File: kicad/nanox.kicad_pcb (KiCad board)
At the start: 4 copper layers, 61.7 x 15.9 mm, 137 parts, among them P1 likely an ESD protection diod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, P2 likely an ESD protection diod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, P3 likely an ESD protection diod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, P4 likely an ESD protection diod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, P5 likely an ESD protection diod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, SW1 push button, left, SW2 push button, right, X1 ?, X10 unknown, marked 1C4F, likely 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, X2 unknown, marked 2GC, X3 unknown, marked 6, X4 ?, X5 ?, X6 ?, X7 ?, X8 ?, X9 unknown, marked P8W 26, Y1 crystal, likely the 32 MHz HSE

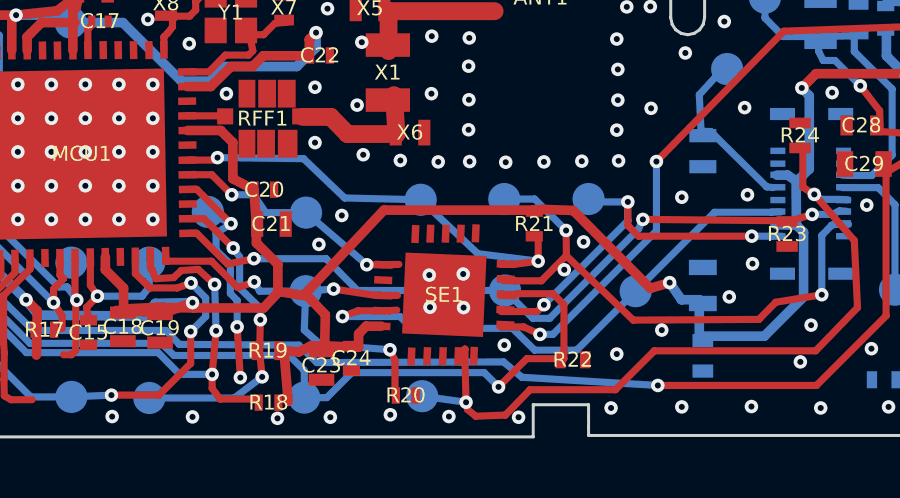
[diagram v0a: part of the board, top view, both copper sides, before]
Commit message: Put the secure element's pads on the real ones, and land its traces on them
The SE outline sat about 0.3 mm left of the real package, so OLED SPI CS
ran down the real pin 9 but stopped beside the modelled one, with a stub
across to it. The outline now follows the pads measured in the bare photo,
and every SE trace ends on its pin's centre with a straight final run;
the CS stub is gone.

Co-Authored-By: Claude Opus 5.5 <noreply@anthropic.com>
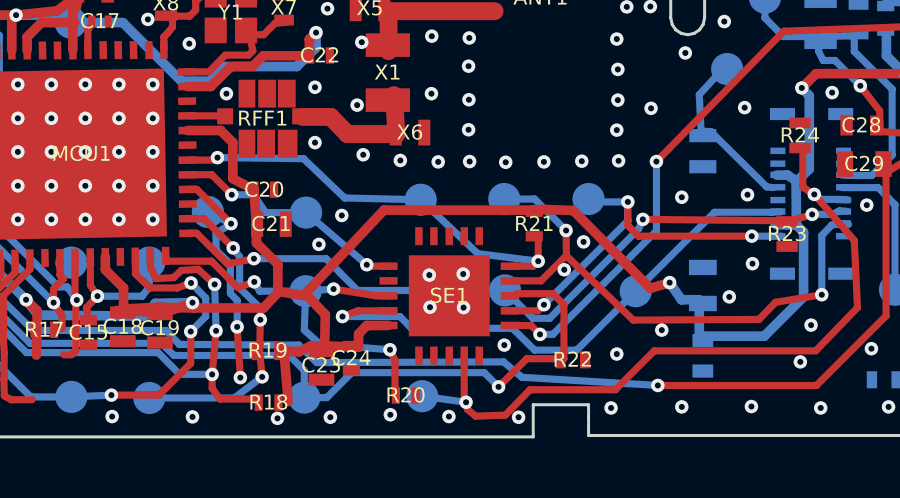
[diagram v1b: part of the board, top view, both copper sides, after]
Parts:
- moved SE1 0.17 mm to (42.0, 22.5)
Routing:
- net OLED SPI CS: track 25.6 -> 25.1 mm
